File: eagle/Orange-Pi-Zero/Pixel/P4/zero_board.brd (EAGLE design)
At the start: 47.8 x 46 mm, 13 parts, among them CN1 1X4-3.5MM, IC1 74HCT125, J1 1X2-3.5MM

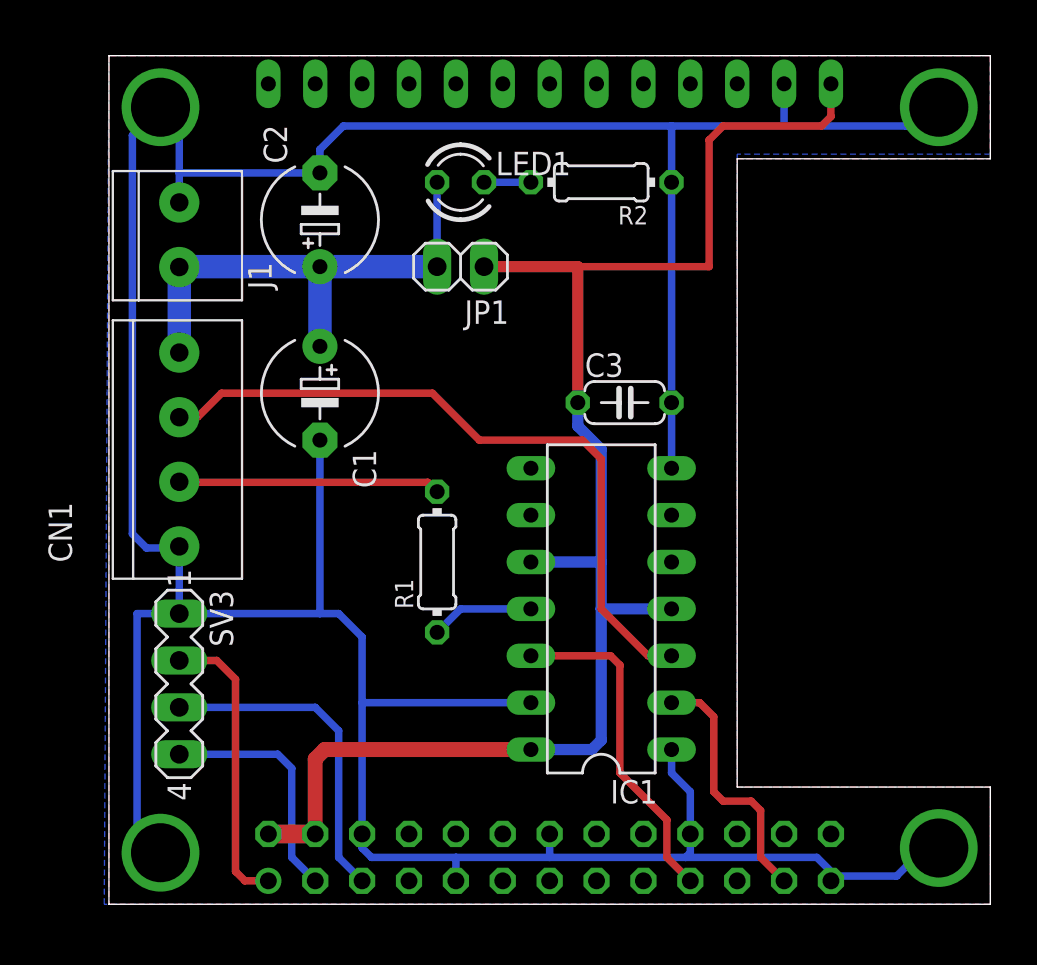
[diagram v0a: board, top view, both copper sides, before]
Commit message: Added new gerber.zip files
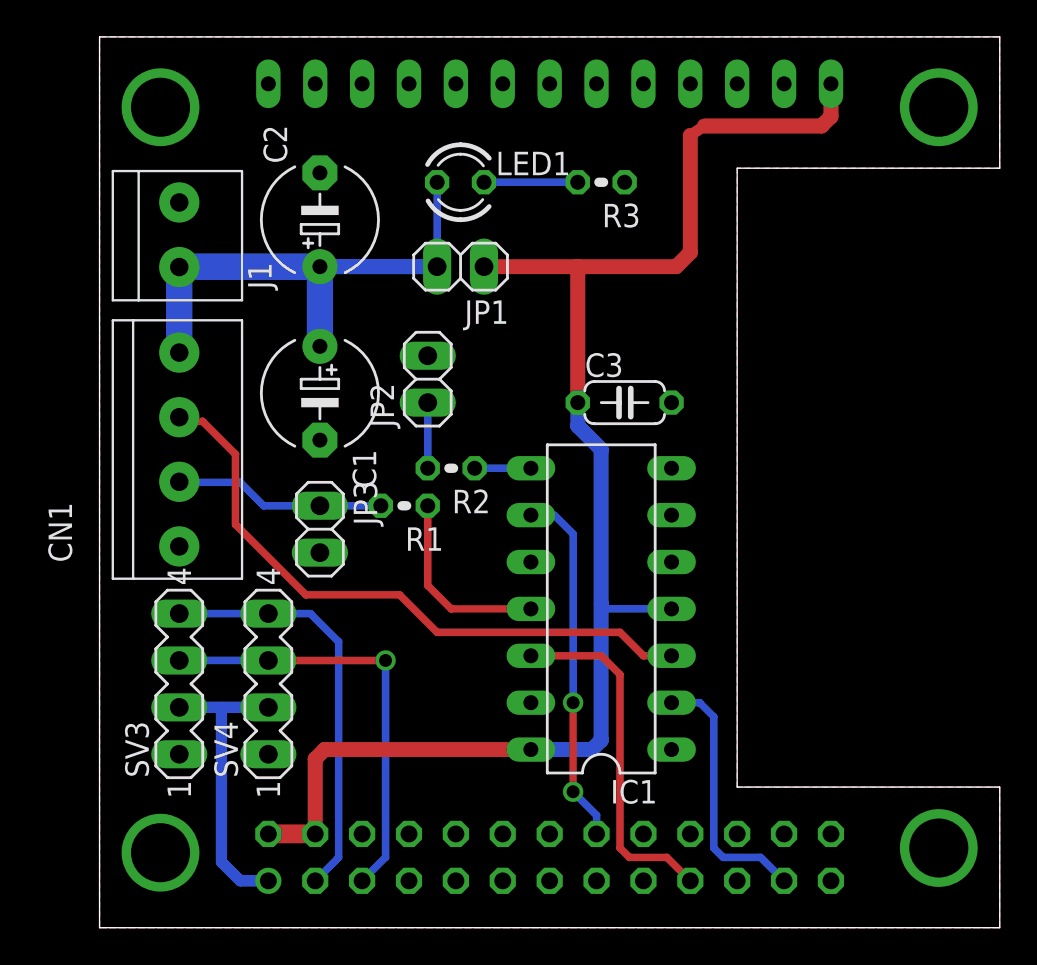
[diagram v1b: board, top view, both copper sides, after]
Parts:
- added JP2: LED EXT, pinhead:1X02
- added JP3: Debug, pinhead:1X02
- added R3: 330, rcl:0204V
- added SV4: I2C-7SEGMENT, con-lstb:MA04-1
- R1, R2: device rcl:0204/7 -> rcl:0204V
- moved R2 17.5 mm to (19.8, 23.4)
- moved R1 3.53 mm to (17.3, 21.3), turned to 180 degrees
- turned SV3 to 90 degrees
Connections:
- removed net N$2: CN1.3, R1.2
- new net N$3: IC1.8, R2.1
- new net N$4: JP2.1, R2.2
- new net OUT: CN1.3, JP3.1, R1.2
- new net STATUS_LED: IC1.9, SV2.16
- net 3V3: now also SV4.2
- net 5V: no longer IC1.10
- net GND: now also IC1.10, JP2.2, JP3.2, R3.1, SV4.1; no longer R2.1
- net I2C_SCL: now also SV4.3
- net I2C_SDA: now also SV4.4
- net N$1: now also R3.2; no longer R2.2
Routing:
- net GND: track 198.1 -> 0.36 mm
- net STATUS_LED: track 0.00 -> 19.5 mm, vias 0 -> 2
- net N$2: track 14.2 -> 0.00 mm
- net OUT: track 0.00 -> 11.5 mm
- net I2C_SDA: track 13.0 -> 22.7 mm
- net I2C_SCL: track 17.8 -> 23.6 mm, vias 0 -> 1
- net MOSI: track 5.61 -> 10.4 mm
- net 5V: track 84.3 -> 80.2 mm
- net CLK: track 37.9 -> 34.3 mm
- net N$4: track 0.00 -> 3.56 mm
- net N$3: track 0.00 -> 3.05 mm
- net N$1: track 2.54 -> 5.08 mm
- net SPI_MOSI: track 18.3 -> 19.2 mm
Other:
- board size 47.8 x 46 mm -> 48.8 x 48.3 mm
